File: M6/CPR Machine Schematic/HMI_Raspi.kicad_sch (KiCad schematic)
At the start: 4 parts, among them J2 Raspberry_Pi_4, SW2 Non-LED Button, SW3 LED Button, SW4 LED Button

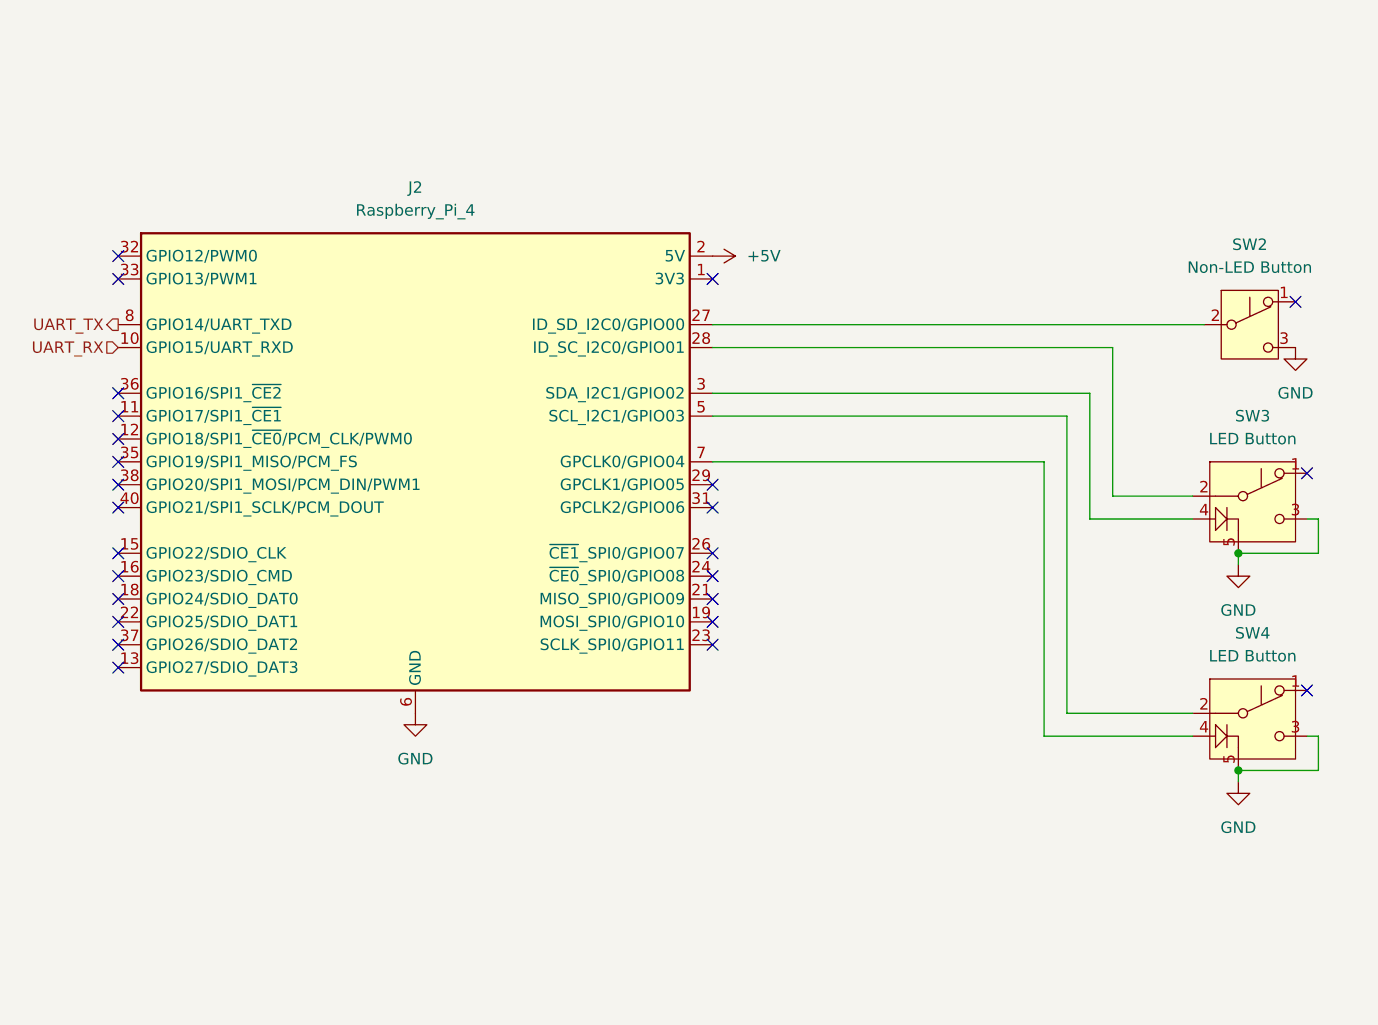
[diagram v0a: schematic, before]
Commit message: Start of Schematic V2
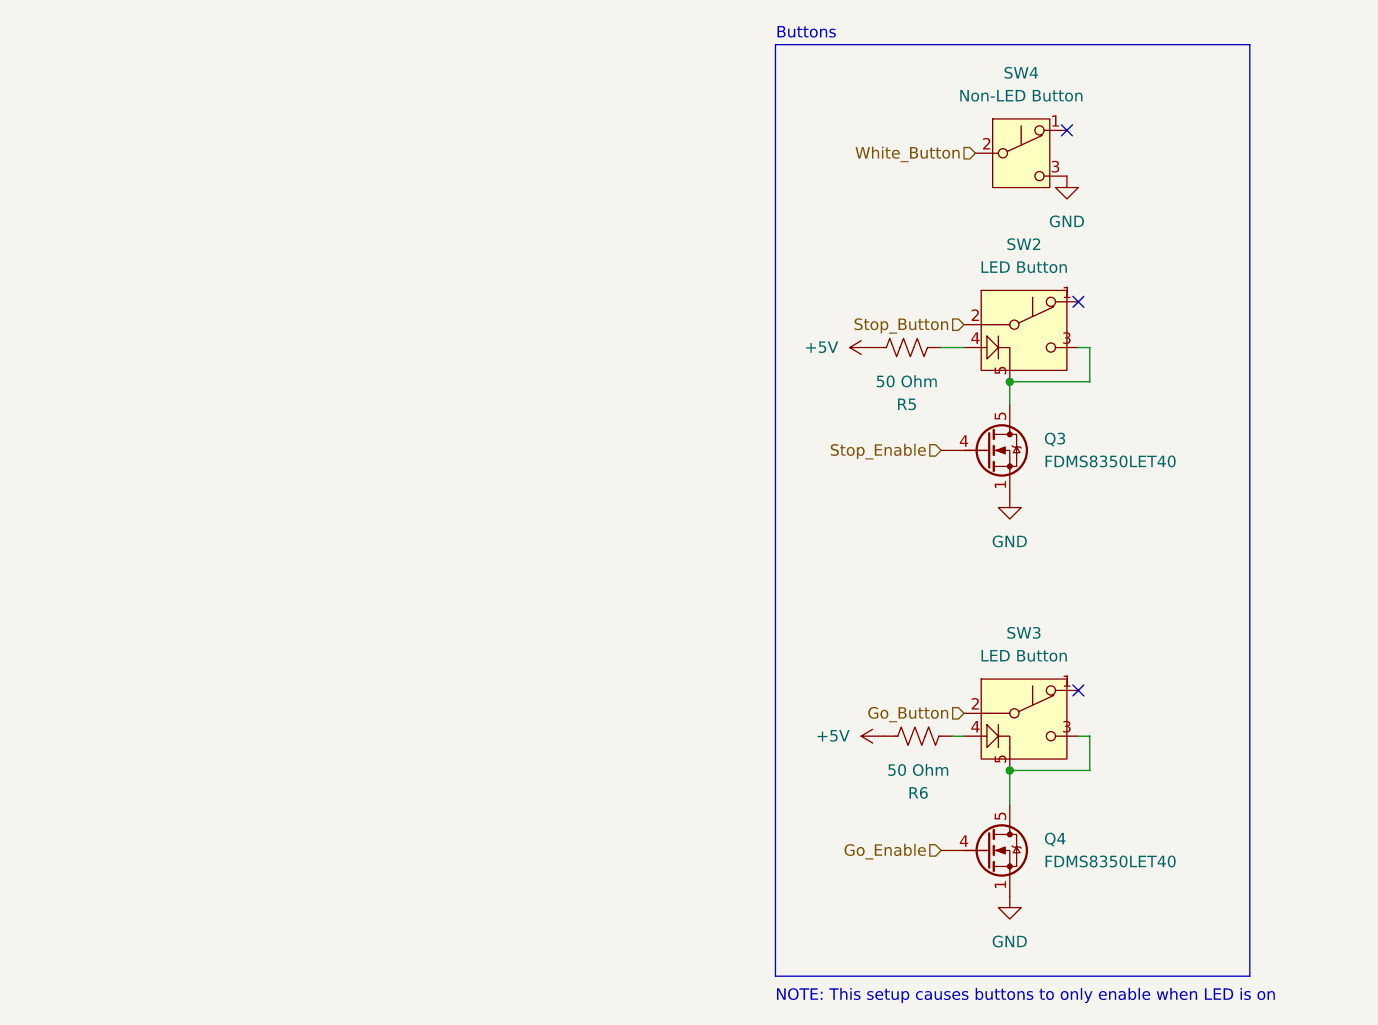
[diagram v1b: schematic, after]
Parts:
- removed J2: Raspberry_Pi_4, symbol Connector:Raspberry_Pi_4
- added Q3, Q4: FDMS8350LET40, Package_TO_SOT_SMD:TDSON-8-1, symbol Transistor_FET:FDMS8350LET40
- added R5, R6: 50 Ohm, symbol Device:R_US
- SW2: value Non-LED Button -> LED Button
- SW4: value LED Button -> Non-LED Button
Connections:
- net +5V: now also R5.2, R6.2
- net GND: now also Q3.1 (S), Q3.2 (S), Q3.3 (S), Q4.1 (S), Q4.2 (S), Q4.3 (S); no longer SW2.3 (C), SW3.3 (C), SW3.5 (GND), SW4.5 (GND)
- net Go_Button: now reaches SW3.2 (B)
- net at SW3.4 (LED_IN): now also R6.1
- net Stop_Button: now reaches SW2.2 (B)
- net White_Button: now reaches SW4.2 (B)
- new net: Q4.5 (D), SW3.3 (C), SW3.5 (GND)
- new net: R5.1, SW2.4 (LED_IN)
- new net: Q3.5 (D), SW2.3 (C), SW2.5 (GND)
- new net Go_Enable: Q4.4 (G)
- new net Stop_Enable: Q3.4 (G)
- no-connect marks 25 -> 3
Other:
- note added: "Buttons"
- note added: "NOTE: This setup causes buttons to only enable when LED is on"

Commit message: More PCB Progress
All Footprints
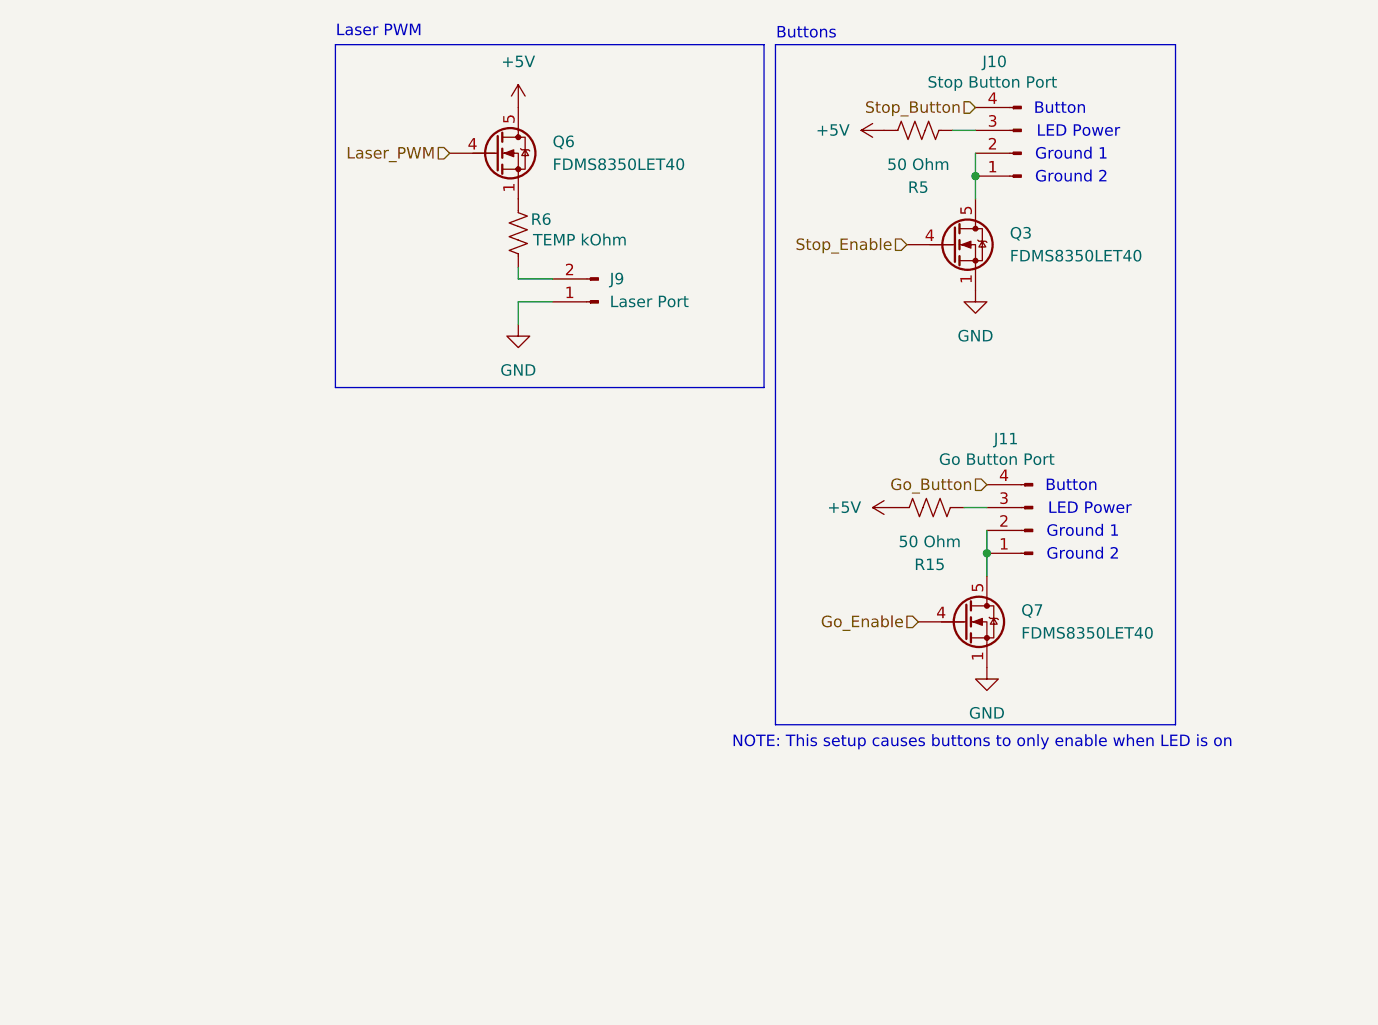
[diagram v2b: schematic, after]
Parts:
- removed Q4: FDMS8350LET40, Package_TO_SOT_SMD:TDSON-8-1, symbol Transistor_FET:FDMS8350LET40
- removed SW2, SW3: LED Button, symbol Switch:SW_Push_SPDT
- removed SW4: Non-LED Button, symbol Switch:SW_Push_SPDT
- added J10: Stop Button Port, Connector_PinHeader_2.54mm:PinHeader_1x04_P2.54mm_Vertical, symbol Connector:Conn_01x04_Pin
- added J11: Go Button Port, Connector_PinHeader_2.54mm:PinHeader_1x04_P2.54mm_Vertical, symbol Connector:Conn_01x04_Pin
- added J9: Laser Port, Connector_PinHeader_2.54mm:PinHeader_1x02_P2.54mm_Vertical, symbol Connector:Conn_01x02_Pin
- added Q6, Q7: FDMS8350LET40, Package_TO_SOT_SMD:TDSON-8-1, symbol Transistor_FET:FDMS8350LET40
- added R15: 50 Ohm, Resistor_SMD:R_1206_3216Metric, symbol Device:R_US
- R5: footprint (none) -> Resistor_SMD:R_1206_3216Metric
- R6: value 50 Ohm -> TEMP kOhm; footprint (none) -> Resistor_SMD:R_1206_3216Metric
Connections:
- net +5V: now also Q6.5 (D), R15.2; no longer R6.2
- net GND: now also J9.1 (Pin_1), Q7.1 (S), Q7.2 (S), Q7.3 (S)
- net Go_Button: now also J11.4 (Pin_4)
- net Go_Enable: now also Q7.4 (G)
- net Stop_Button: now also J10.4 (Pin_4)
- net at R6.1: now also J9.2 (Pin_2)
- net at R5.1: now also J10.3 (Pin_3)
- net at Q3.5 (D): now also J10.1 (Pin_1), J10.2 (Pin_2)
- new net: J11.1 (Pin_1), J11.2 (Pin_2), Q7.5 (D)
- new net: J11.3 (Pin_3), R15.1
- new net: Q6.1 (S), Q6.2 (S), Q6.3 (S), R6.2
- new net Laser_PWM: Q6.4 (G)
- no-connect marks 3 -> 0
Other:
- note added: "Button"
- note added: "Ground 1"
- note added: "Ground 2"
- note added: "LED Power"
- note added: "Laser PWM"
- moved on the sheet: Q3, R5

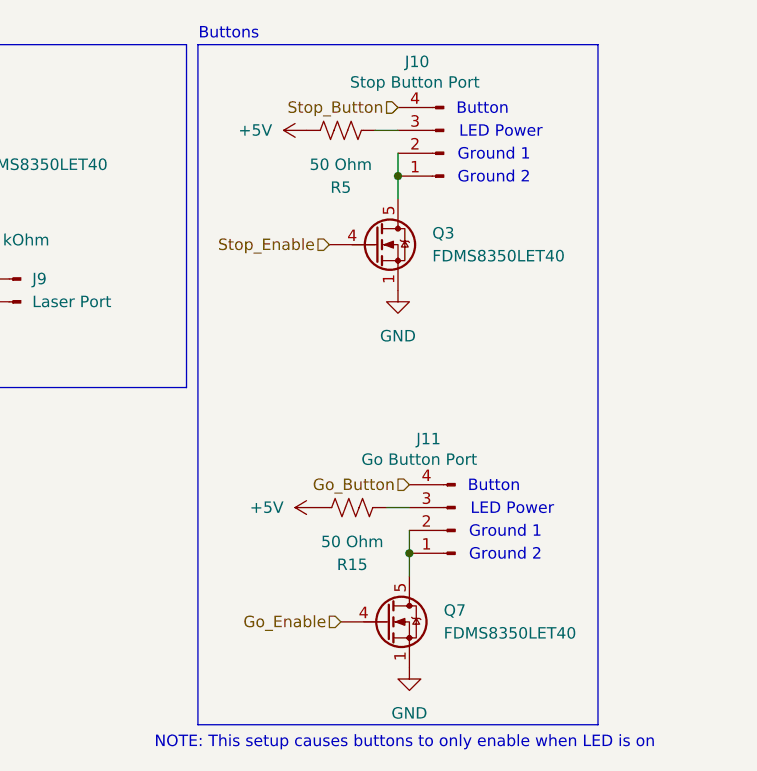
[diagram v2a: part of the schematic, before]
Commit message: finished PCB Draft
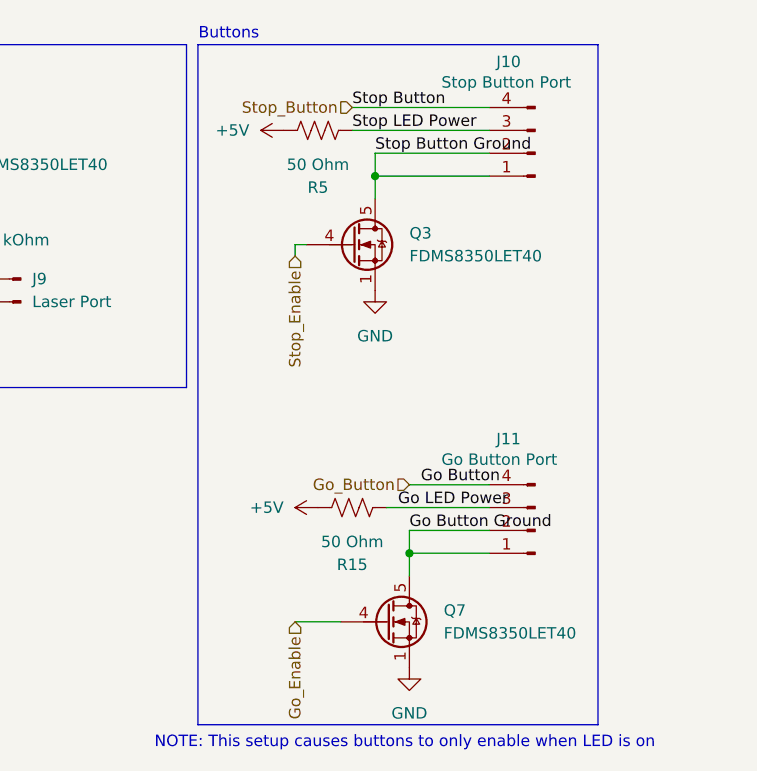
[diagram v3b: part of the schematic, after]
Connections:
- net Stop Button Ground: now reaches J10.1 (Pin_1), J10.2 (Pin_2), Q3.5 (D)
- net Stop LED Power: now reaches J10.3 (Pin_3), R5.1
- net Go Button Ground: now reaches J11.1 (Pin_1), J11.2 (Pin_2), Q7.5 (D)
- net Go LED Power: now reaches J11.3 (Pin_3), R15.1
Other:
- note removed: "Button"
- note removed: "Ground 1"
- note removed: "Ground 2"
- note removed: "LED Power"
- moved on the sheet: J10, J11, Q3, R5

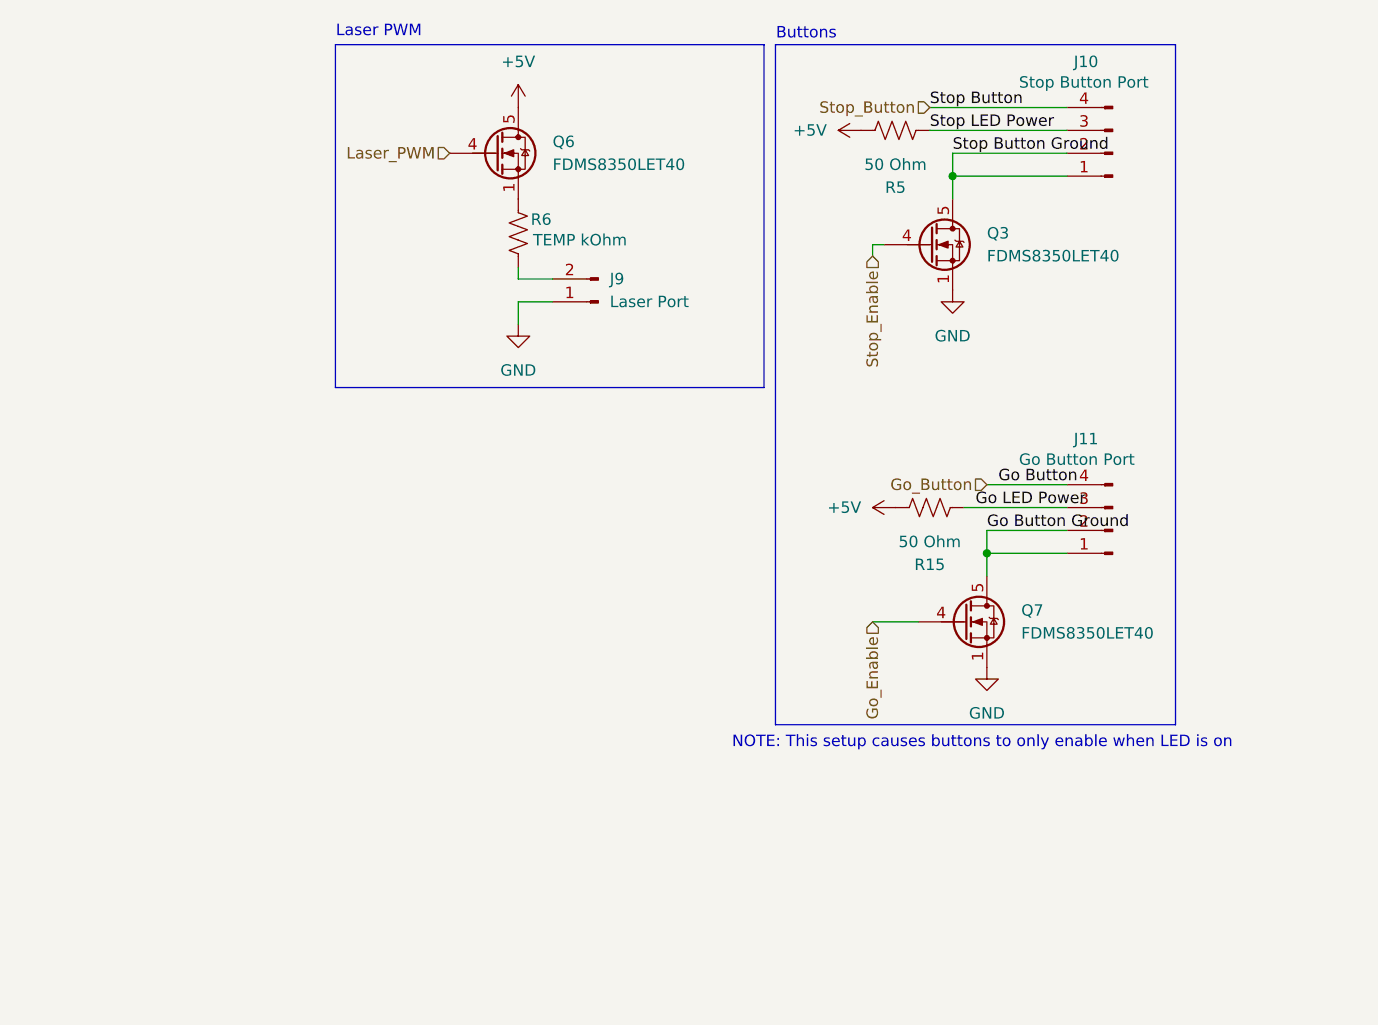
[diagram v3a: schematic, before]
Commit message: PCB Feedback V1
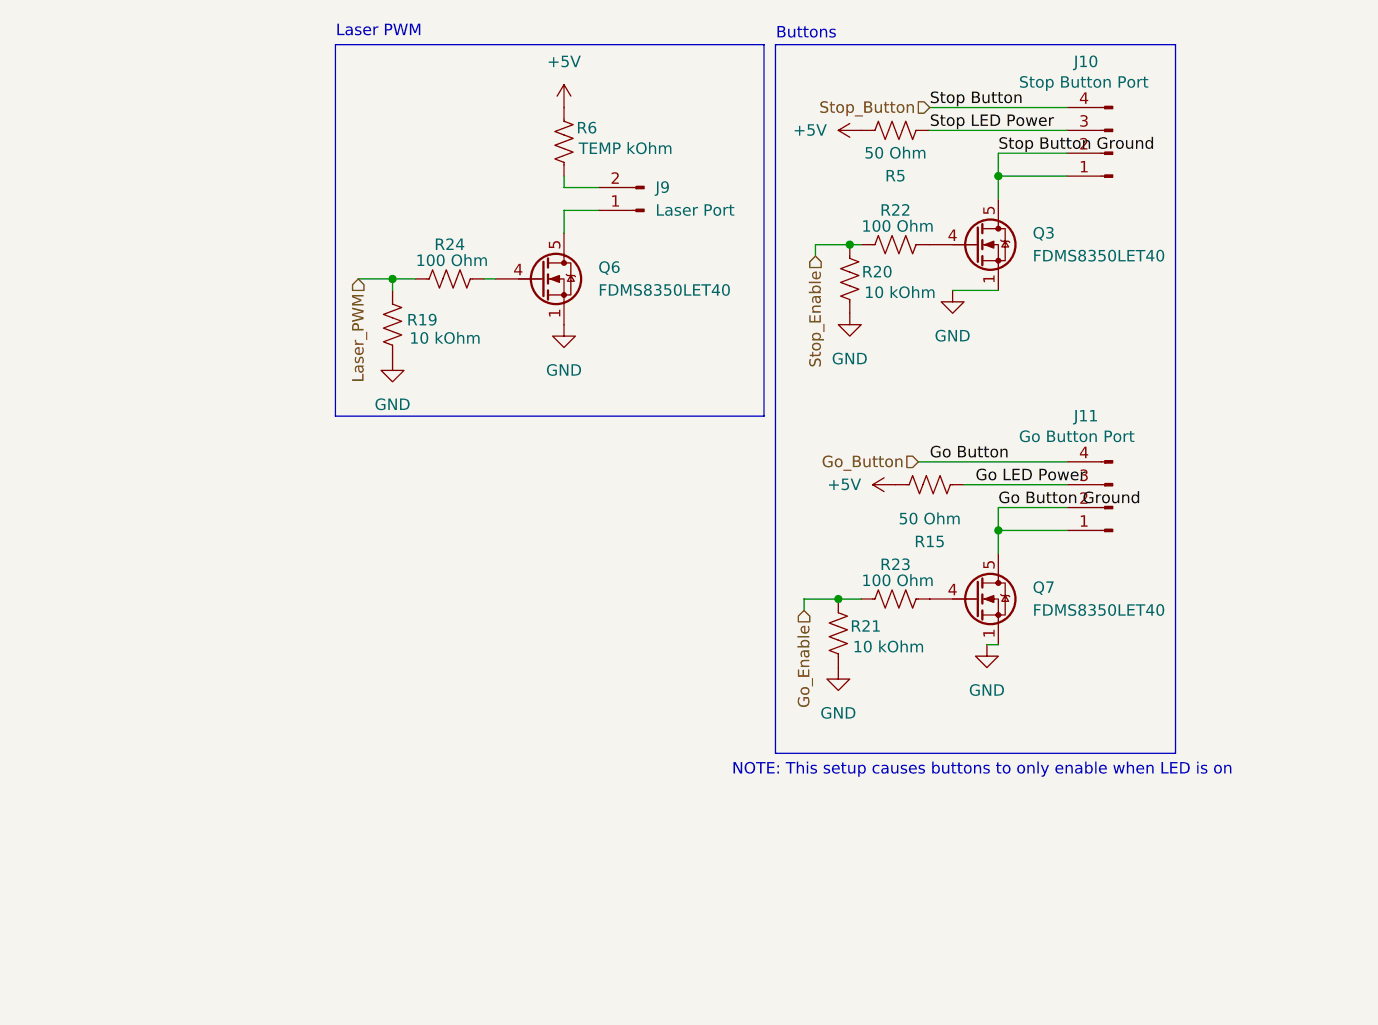
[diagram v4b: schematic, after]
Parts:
- added R19, R20, R21: 10 kOhm, Resistor_SMD:R_1206_3216Metric, symbol Device:R_US
- added R22, R23, R24: 100 Ohm, Resistor_SMD:R_1206_3216Metric, symbol Device:R_US
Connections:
- net +5V: now also R6.2; no longer Q6.5 (D)
- net GND: now also Q6.1 (S), Q6.2 (S), Q6.3 (S), R19.2, R20.2, R21.2; no longer J9.1 (Pin_1)
- net Go_Enable: now also R21.1, R23.1; no longer Q7.4 (G)
- net Laser_PWM: now also R19.1, R24.1; no longer Q6.4 (G)
- net Stop_Enable: now also R20.1, R22.1; no longer Q3.4 (G)
- new net: J9.1 (Pin_1), Q6.5 (D)
- new net: Q3.4 (G), R22.2
- new net: Q7.4 (G), R23.2
- new net: Q6.4 (G), R24.2
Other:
- moved on the sheet: J11, J9, Q3, Q6, Q7, R15, R6
